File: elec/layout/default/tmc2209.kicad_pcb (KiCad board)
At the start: 2 copper layers, 225.7 x 100.8 mm, 0 parts

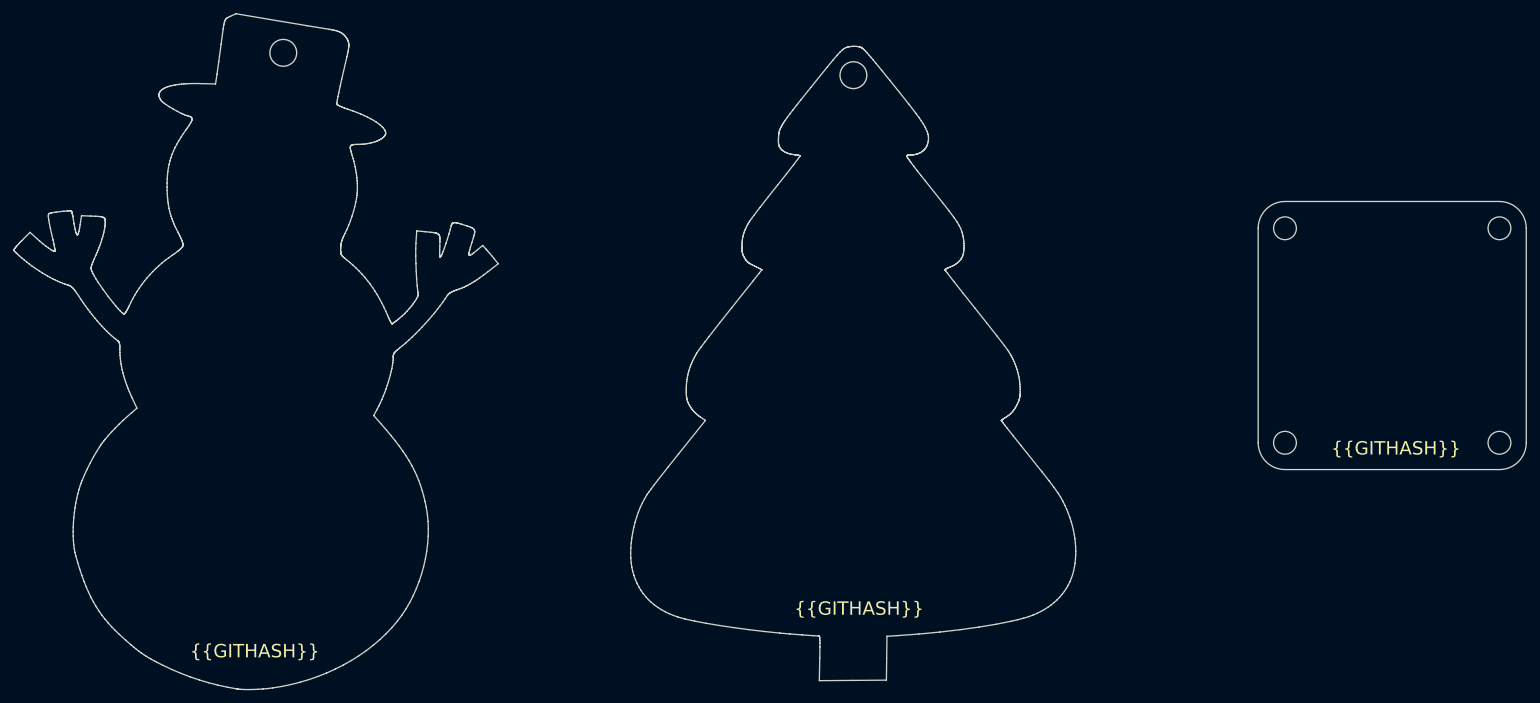
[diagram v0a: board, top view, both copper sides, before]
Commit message: added layout
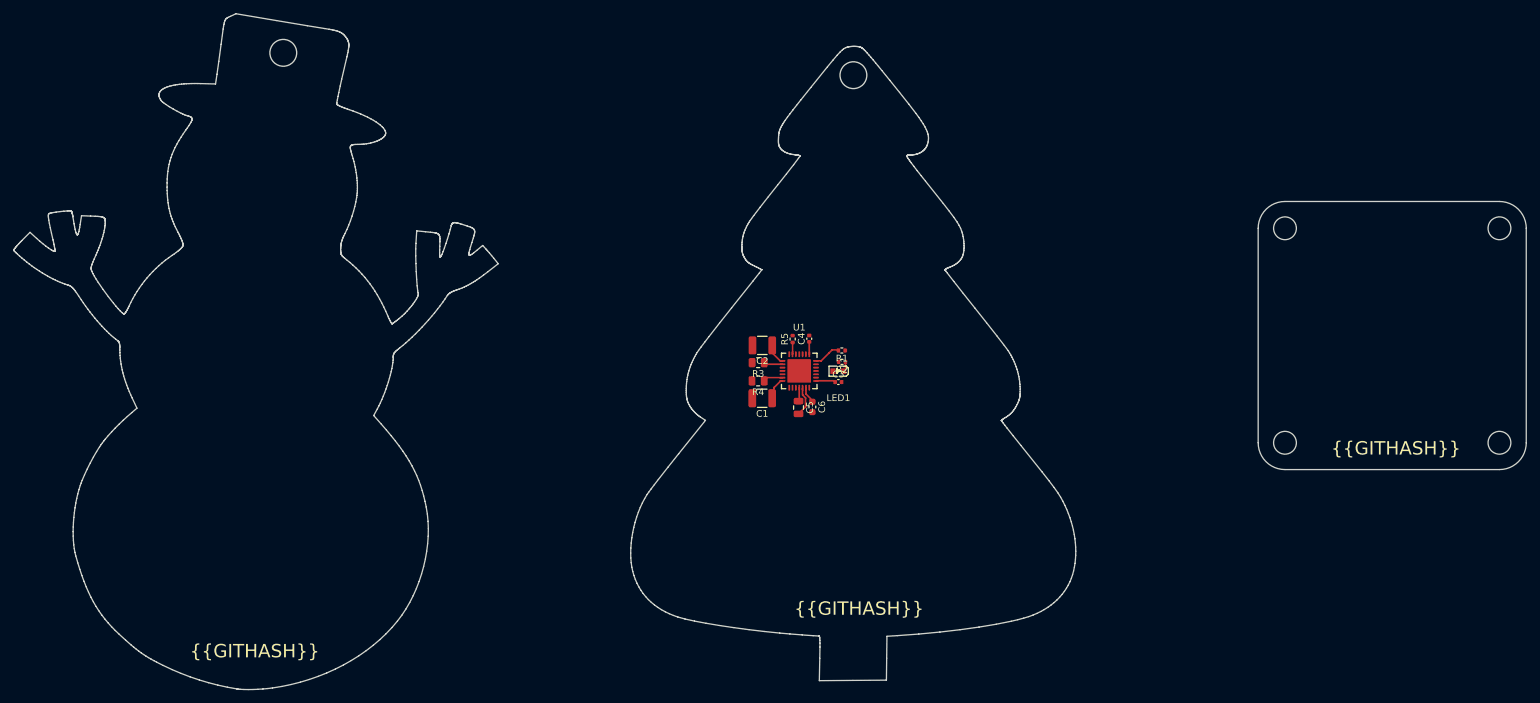
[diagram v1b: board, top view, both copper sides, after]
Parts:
- added C1: Multilayer Ceramic Capacitors MLCC - SMD/SMT 2.2uF 100V 121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, lib:C1210, F.Cu at (147.6, 107.1)
- added C2: Multilayer Ceramic Capacitors MLCC - SMD/SMT 2.2uF 100V 121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, lib:C1210, F.Cu at (147.6, 99.3)
- added C3: Multilayer Ceramic Capacitors MLCC - SMD/SMT 2.2uF 16V 0402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, lib:C0402, F.Cu at (159.0, 104.7)
- added C4: Multilayer Ceramic Capacitors MLCC - SMD/SMT 100nF 10V 0402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, lib:C0402, F.Cu at (154.6, 98.3)
- added C5: Multilayer Ceramic Capacitors MLCC - SMD/SMT 22nF 50V 0805 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, lib:C0805, F.Cu at (153.0, 108.5)
- added C6: Multilayer Ceramic Capacitors MLCC - SMD/SMT 100nF 50V 0603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, lib:C0603, F.Cu at (155.1, 108.4)
- added LED1: , lib:LED0603-RD, F.Cu at (159.0, 103.1)
- added R1: Chip Resistor - Surface Mount 1.1KOhms ±5% 1/16W 0402 RoHS, lib:R0402, F.Cu at (159.5, 100.0)
- added R2: Chip Resistor - Surface Mount 120Ohms ±5% 1/16W 0402 RoHS, lib:R0402, F.Cu at (159.5, 101.7)
- added R3: Chip Resistor - Surface Mount 0.12Ohms ±5% 1/8W 0805 RoHS, lib:R0805, F.Cu at (147.0, 101.8)
- added R4: Chip Resistor - Surface Mount 0.12Ohms ±5% 1/8W 0805 RoHS, lib:R0805, F.Cu at (147.0, 104.6)
- added R5: Chip Resistor - Surface Mount 110KOhms ±5% 1/16W 0402 RoHS, lib:R0402, F.Cu at (152.2, 98.3)
- added U1: , lib:QFN-28_L5.0-W5.0-P0.50-BL-EP, F.Cu at (153.1, 103.1)
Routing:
- net vcc: track 0.00 -> 5.93 mm
- net cpi: track 0.00 -> 4.53 mm
- net pdn_uart: track 0.00 -> 4.06 mm
- net _5vout: track 0.00 -> 2.96 mm
- net bra: track 0.00 -> 2.53 mm
- net brb: track 0.00 -> 2.51 mm
- net vcp: track 0.00 -> 2.49 mm
- net cpo: track 0.00 -> 2.05 mm
- net vcc_io: track 0.00 -> 1.83 mm
- net stdby: track 0.00 -> 1.75 mm
- net cathode: track 0.00 -> 1.49 mm
